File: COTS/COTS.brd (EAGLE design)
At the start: 90.2 x 100 mm, 9 parts

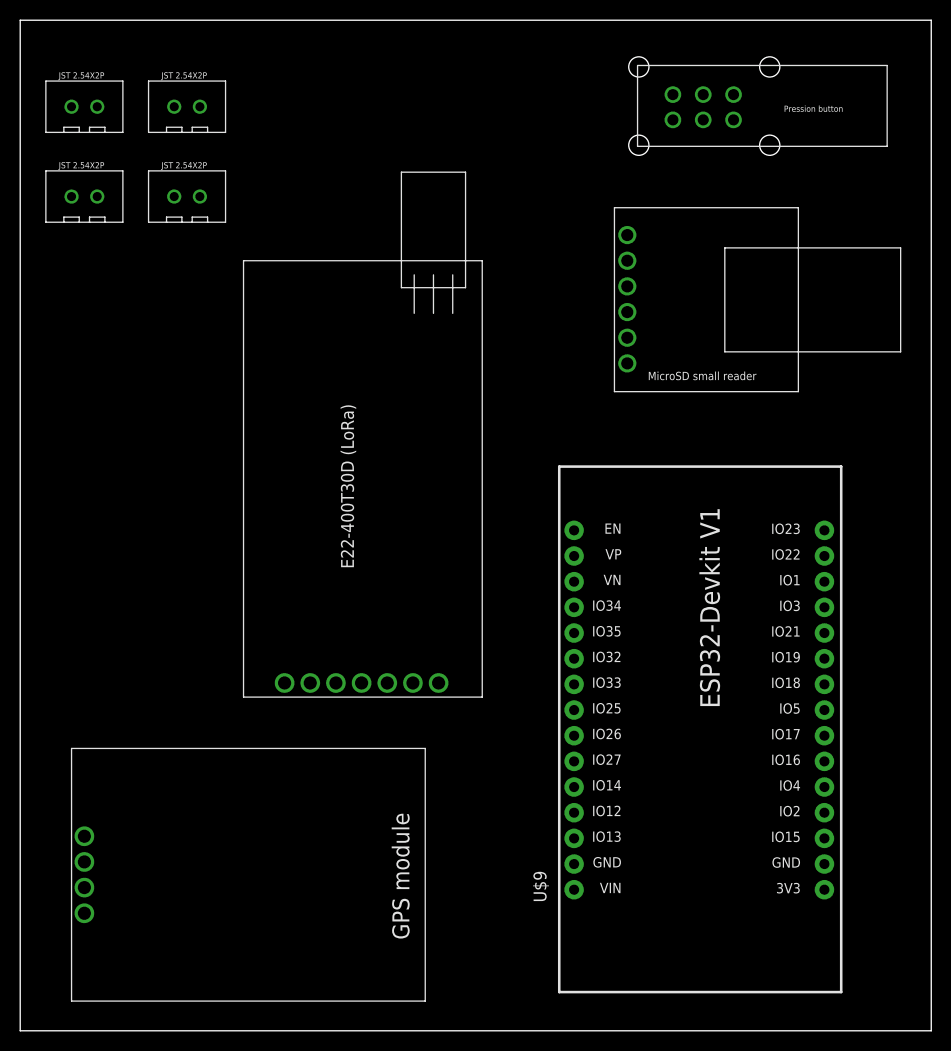
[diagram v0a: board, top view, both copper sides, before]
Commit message: Update
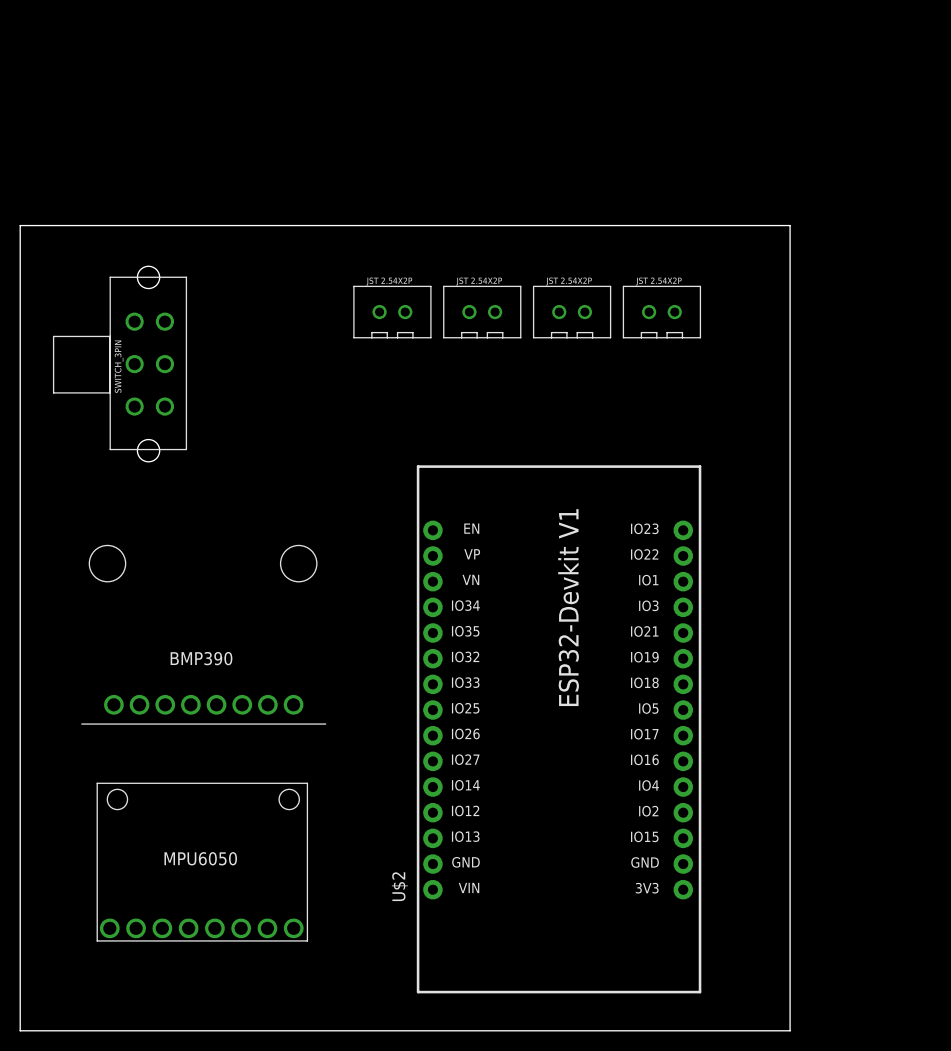
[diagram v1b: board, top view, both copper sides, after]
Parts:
- removed U$9: ESP32DEVKITV1, ESP32-DEVKITV1:ESP32-DEVKITV1
- U$1: value PRESSION_BUTTON -> MPU6050V1; device CRD:PRESSION_BUTTON_FOOTPRINT -> CRD:MPU6050_FOOTPRINT
- U$2: value MICROSD_SMALL_READER -> ESP32DEVKITV1; device CRD:MICROSD_SMALL_READER_FOOTPRINT -> ESP32-DEVKITV1:ESP32-DEVKITV1
- U$3: value JST2.54X2P -> BMP390V1; device CRD:JST2.54X2P_FOOTPRINT -> CRD:BMP390_FOOTPRINT
- U$7: value GPS_MODULE -> JST2.54X2P; device CRD:GPS_MODULE_FOOTPRINT -> CRD:JST2.54X2P_FOOTPRINT
- U$8: value E22-400T30D -> SWITCH_3PIN; device CRD:E22-400T30D_FOOTPRINT -> CRD:SWITCH_3PIN_FOOTPRINT
- moved U$1 89.7 mm to (17.8, 20.3)
- moved U$6 58.3 mm to (63.5, 71.1)
- moved U$7 57.6 mm to (36.8, 71.1), turned to 0 degrees
- moved U$3 52.1 mm to (17.8, 40.6)
- moved U$4 39.8 mm to (54.6, 71.1)
- moved U$2 38.7 mm to (52.1, 36.8), turned to 90 degrees
- moved U$5 35.6 mm to (45.7, 71.1)
- moved U$8 27.5 mm to (12.7, 66.0)
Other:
- board size 90.2 x 100 mm -> 76.2 x 79.7 mm
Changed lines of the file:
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@@
 </layers>
 <board>
-<fusionsync huburn="a.YnVzaW5lc3M6ZGlzY2VudGUxNzg" projecturn="a.YnVzaW5lc3M6ZGlzY2VudGUxNzgjRDIwMjIwNjExNTMyNjQzNTAx" f3durn="urn:adsk.wipprod:dm.lineage:LO0rVtrmTNmc-QnwxbZBTA" pcbguid="9d58484e-0a02-4060-8550-79589bd949fc" lastpulledtime="" lastsyncedchangeguid="" latestrevisionid="46605ec0-6288-40dc-83f6-c90f963cb555" lastsyncedrevisionid="46605ec0-6288-40dc-83f6-c90f963cb555" lastboardhashguid="0044dba3-1b92-d3f1-3d10-6736c9c82925" lastpushedtime="2024-04-18T17:53:33Z" linktopcb3d="true"/>
 <plain>
-<wire x1="0" y1="0" x2="90.15" y2="0" width="0" layer="20"/>
-<wire x1="90.15" y1="0" x2="90.15" y2="100" width="0" layer="20"/>
-<wire x1="90.15" y1="100" x2="0" y2="100" width="0" layer="20"/>
-<wire x1="0" y1="100" x2="0" y2="0" width="0" layer="20"/>
-<dimension x1="-2.54" y1="0" x2="-2.54" y2="100.33" x3="-6.35" y3="50.165" textsize="1.778" layer="47"/>
-<dimension x1="0" y1="-3.81" x2="90.17" y2="-3.81" x3="45.085" y3="-6.35" textsize="1.778" layer="47"/>
+<wire x1="0" y1="0" x2="76.18" y2="0" width="0" layer="20"/>
+<wire x1="76.18" y1="0" x2="76.18" y2="79.68" width="0" layer="20"/>
+<wire x1="76.18" y1="79.68" x2="0" y2="79.68" width="0" layer="20"/>
+<wire x1="0" y1="79.68" x2="0" y2="0" width="0" layer="20"/>
+<dimension x1="-3.81" y1="0" x2="-3.81" y2="90.17" x3="-7.62" y3="45.085" textsize="1.778" layer="47"/>
+<dimension x1="0" y1="-5.08" x2="100.33" y2="-5.08" x3="50.165" y3="-8.89" textsize="1.778" layer="47"/>
 </plain>
 <attributes>
@@
 </autorouter>
 <elements>
-<element name="U$1" library="CRD" library_urn="urn:adsk.eagle:library:39051337" package="PRESSION_BUTTON_FOOTPRINT" package3d_urn="urn:adsk.eagle:package:43483815/3" value="PRESSION_BUTTON" x="72.39" y="91.44" smashed="yes"/>
-<element name="U$2" library="CRD" library_urn="urn:adsk.eagle:library:39051337" package="MICROSD_SMALL_READER_FOOTPRINT" package3d_urn="urn:adsk.eagle:package:44017969/2" value="MICROSD_SMALL_READER" x="67.31" y="72.39" smashed="yes"/>
-<element name="U$3" library="CRD" library_urn="urn:adsk.eagle:library:39051337" package="JST2.54X2P_FOOTPRINT" package3d_urn="urn:adsk.eagle:package:39191967/2" value="JST2.54X2P" x="6.35" y="91.44" smashed="yes"/>
-<element name="U$4" library="CRD" library_urn="urn:adsk.eagle:library:39051337" package="JST2.54X2P_FOOTPRINT" package3d_urn="urn:adsk.eagle:package:39191967/2" value="JST2.54X2P" x="16.51" y="82.55" smashed="yes"/>
-<element name="U$5" library="CRD" library_urn="urn:adsk.eagle:library:39051337" package="JST2.54X2P_FOOTPRINT" package3d_urn="urn:adsk.eagle:package:39191967/2" value="JST2.54X2P" x="16.51" y="91.44" smashed="yes"/>
-<element name="U$6" library="CRD" library_urn="urn:adsk.eagle:library:39051337" package="JST2.54X2P_FOOTPRINT" package3d_urn="urn:adsk.eagle:package:39191967/2" value="JST2.54X2P" x="6.35" y="82.55" smashed="yes"/>
-<element name="U$7" library="CRD" library_urn="urn:adsk.eagle:library:39051337" package="GPS_MODULE_FOOTPRINT" package3d_urn="urn:adsk.eagle:package:39608400/5" value="GPS_MODULE" x="22.86" y="15.24" smashed="yes" rot="R270"/>
-<element name="U$8" library="CRD" library_urn="urn:adsk.eagle:library:39051337" package="E22-400T30D_FOOTPRINT" package3d_urn="urn:adsk.eagle:package:40965099/4" value="E22-400T30D" x="35.56" y="50.8" smashed="yes" rot="R90"/>
-<element name="U$9" library="ESP32-DEVKITV1" library_urn="urn:adsk.eagle:library:44018017" package="ESP32-DEVKITV1" package3d_urn="urn:adsk.eagle:package:44018021/1" value="ESP32DEVKITV1" x="66.04" y="36.83" smashed="yes" rot="R90">
-<attribute name="NAME" x="52.07" y="12.7" size="1.27" layer="21" rot="R90"/>
+<element name="U$1" library="CRD" library_urn="urn:adsk.eagle:library:39051337" package="MPU6050_FOOTPRINT" package3d_urn="urn:adsk.eagle:package:39029071/8" value="MPU6050V1" x="17.78" y="20.32" smashed="yes"/>
+<element name="U$2" library="ESP32-DEVKITV1" library_urn="urn:adsk.eagle:library:44018017" package="ESP32-DEVKITV1" package3d_urn="urn:adsk.eagle:package:44018021/1" value="ESP32DEVKITV1" x="52.07" y="36.83" smashed="yes" rot="R90">
+<attribute name="NAME" x="38.1" y="12.7" size="1.27" layer="21" rot="R90"/>
 </element>
+<element name="U$3" library="CRD" library_urn="urn:adsk.eagle:library:39051337" package="BMP390_FOOTPRINT" package3d_urn="urn:adsk.eagle:package:40965124/5" value="BMP390V1" x="17.78" y="40.64" smashed="yes"/>
+<element name="U$4" library="CRD" library_urn="urn:adsk.eagle:library:39051337" package="JST2.54X2P_FOOTPRINT" package3d_urn="urn:adsk.eagle:package:39191967/2" value="JST2.54X2P" x="54.61" y="71.12" smashed="yes"/>
+<element name="U$5" library="CRD" library_urn="urn:adsk.eagle:library:39051337" package="JST2.54X2P_FOOTPRINT" package3d_urn="urn:adsk.eagle:package:39191967/2" value="JST2.54X2P" x="45.72" y="71.12" smashed="yes"/>
+<element name="U$6" library="CRD" library_urn="urn:adsk.eagle:library:39051337" package="JST2.54X2P_FOOTPRINT" package3d_urn="urn:adsk.eagle:package:39191967/2" value="JST2.54X2P" x="63.5" y="71.12" smashed="yes"/>
+<element name="U$7" library="CRD" library_urn="urn:adsk.eagle:library:39051337" package="JST2.54X2P_FOOTPRINT" package3d_urn="urn:adsk.eagle:package:39191967/2" value="JST2.54X2P" x="36.83" y="71.12" smashed="yes"/>
+<element name="U$8" library="CRD" library_urn="urn:adsk.eagle:library:39051337" package="SWITCH_3PIN_FOOTPRINT" package3d_urn="urn:adsk.eagle:package:39192263/8" value="SWITCH_3PIN" x="12.7" y="66.04" smashed="yes" rot="R90"/>
 </elements>
 <signals>
@@
 </note>
 <note version="8.3" severity="warning">
-Since Version 8.3, EAGLE supports Fusion synchronisation.
-This feature will not be available in this version and saving
-the document will break the link to the Fusion PCB feature.
-</note>
-<note version="8.3" severity="warning">
